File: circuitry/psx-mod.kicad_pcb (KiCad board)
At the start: 2 copper layers, 57 parts, among them J1 2x3P, J2 1x6P, J3 1x6P, J4 1x6P, J5 USB 2.0 Type-C, Q1 SI2302, Q2 SI2302, SW1 RESET, U1 TPS78318DDCT, U2 CDCE925PWR, U3 74HC04, U4 ATmega328P-A, U5 USBLC6-2SC6, U6 CH340G, Y1 16MHz, Y2 27MHz, Y3 12MHz

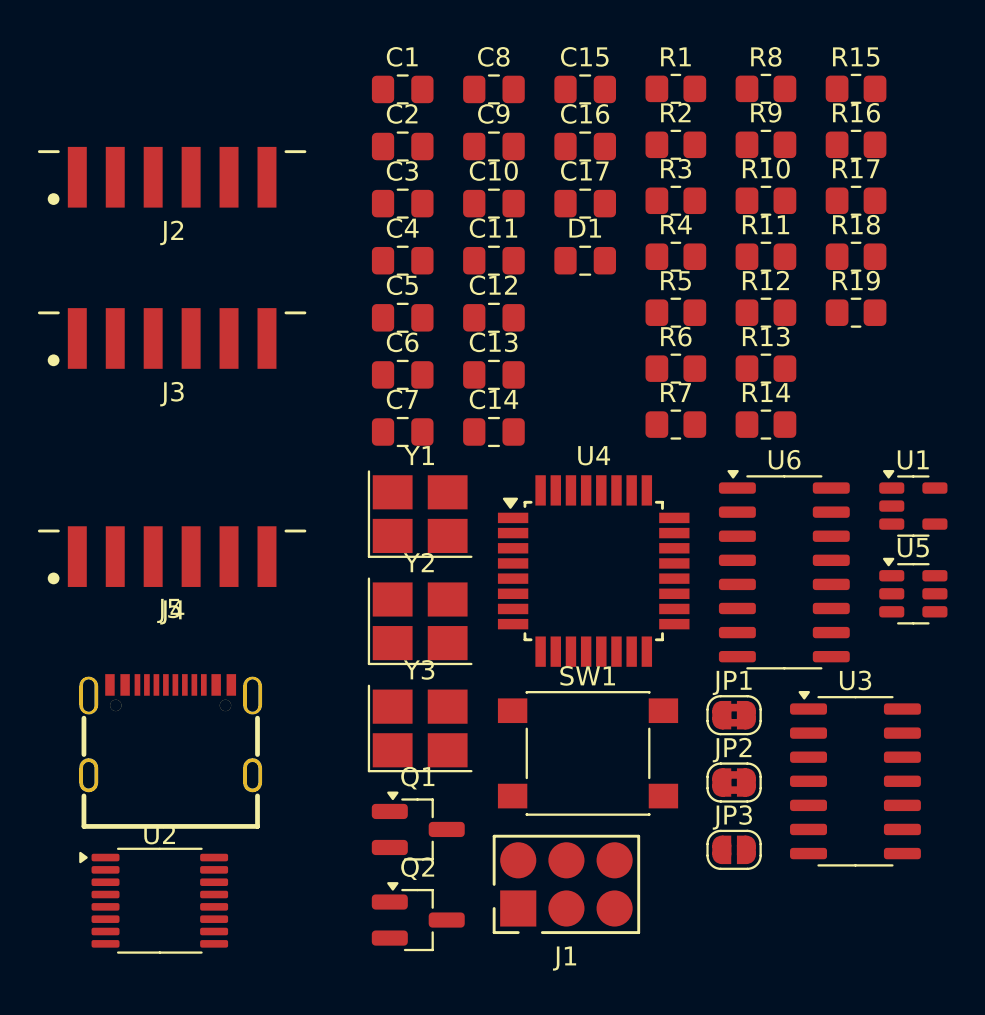
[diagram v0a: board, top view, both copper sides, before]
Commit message: Completed schematic and layout (badly).
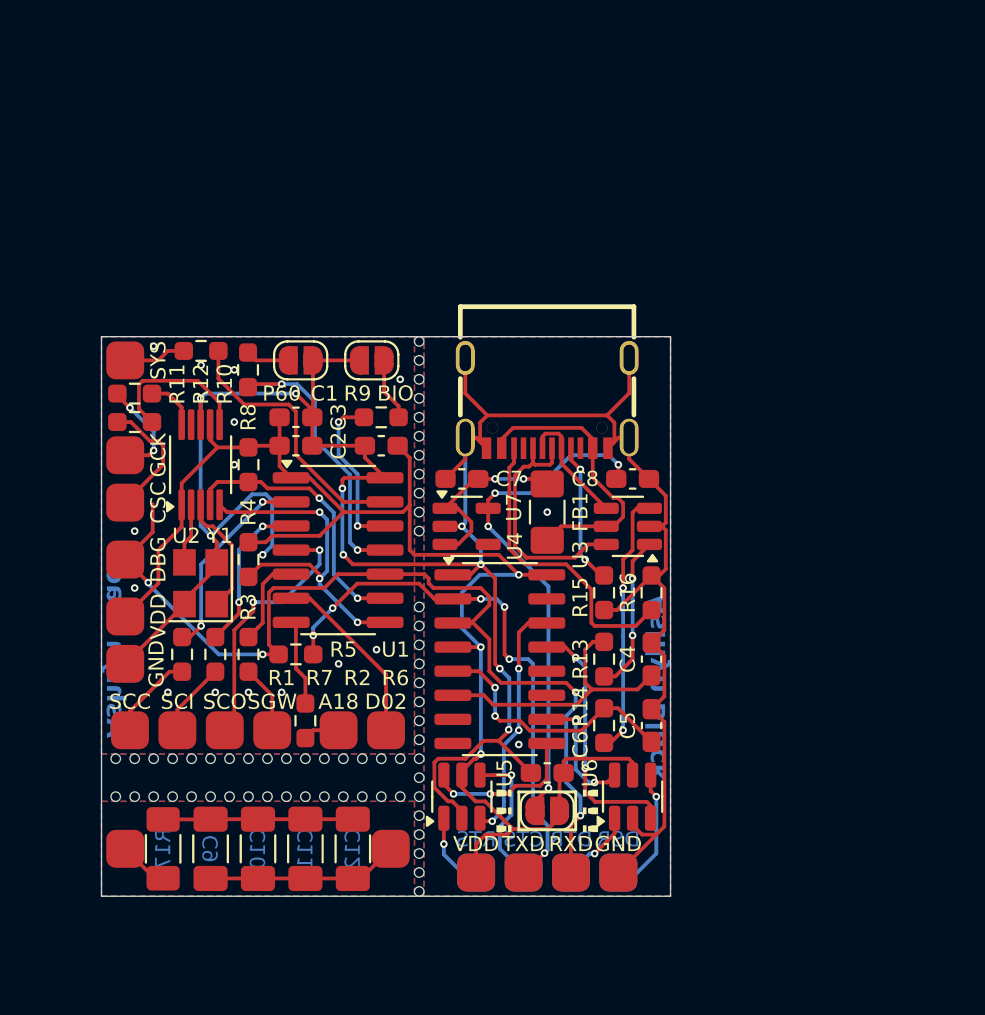
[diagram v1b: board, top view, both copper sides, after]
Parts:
- removed C13, C16: C, Capacitor_SMD:C_0805_2012Metric_Pad1.18x1.45mm_HandSolder
- removed C14, C15: 10pF, Capacitor_SMD:C_0805_2012Metric_Pad1.18x1.45mm_HandSolder
- removed C17: 100nF, Capacitor_SMD:C_0805_2012Metric_Pad1.18x1.45mm_HandSolder
- removed D1: RED, Capacitor_SMD:C_0805_2012Metric_Pad1.18x1.45mm_HandSolder
- removed J2, J3: 1x6P, PSX_Mod:CONN-PH 1x06_P2.00mm_Horizontal
- removed Q1, Q2: SI2302, Package_TO_SOT_SMD:SOT-23_Handsoldering
- removed R18, R19: 5.1kΩ, Resistor_SMD:R_0805_2012Metric_Pad1.20x1.40mm_HandSolder
- removed SW1: RESET, Button_Switch_SMD:SW_Push_1P1T_NO_6x6mm_H9.5mm
- removed Y2: 27MHz, Crystal:Crystal_SMD_3225-4Pin_3.2x2.5mm_HandSoldering
- removed Y3: 12MHz, Crystal:Crystal_SMD_3225-4Pin_3.2x2.5mm_HandSoldering
- added FB1: FerriteBead, Inductor_SMD:L_1206_3216Metric_Pad1.42x1.75mm_HandSolder, F.Cu at (158.8, 98.0)
- added J10: USB 2.0 Type-C, PSX_Mod:CONN-SMD_HX-TYPE-C-16PIN, F.Cu at (158.8, 92.2)
- added J11: Conn_01x04, PSX_Mod:CONN-SMD_4P, B.Cu at (158.8, 117.0)
- added J12: Conn_01x01, PSX_Mod:CONN-SMD_1P, F.Cu at (136.5, 115.8)
- added J13: Conn_01x01, PSX_Mod:CONN-SMD_1P, F.Cu at (150.5, 115.8)
- added J6: Conn_01x01, PSX_Mod:CONN-SMD_1P, F.Cu at (136.5, 100.5)
- added J7: Conn_01x01, PSX_Mod:CONN-SMD_1P, F.Cu at (136.5, 90.0)
- added J8: Conn_01x02, PSX_Mod:CONN-SMD_2P, F.Cu at (136.5, 96.2)
- added J9: Conn_01x04, PSX_Mod:CONN-SMD_4P, F.Cu at (158.8, 117.0)
- added REF**: MouseBite, PSX_Mod:MouseBite, F.Cu at (141.0, 113.0)
- added REF**: MouseBite, PSX_Mod:MouseBite, F.Cu at (147.0, 113.0)
- added REF**: MouseBite, PSX_Mod:MouseBite, F.Cu at (152.0, 90.0)
- added REF**: MouseBite, PSX_Mod:MouseBite, F.Cu at (152.0, 115.0)
- added REF**: MouseBite, PSX_Mod:MouseBite, F.Cu at (152.0, 114.0)
- added REF**: MouseBite, PSX_Mod:MouseBite, F.Cu at (152.0, 112.0)
- added REF**: MouseBite, PSX_Mod:MouseBite, F.Cu at (149.0, 111.0)
- added REF**: MouseBite, PSX_Mod:MouseBite, F.Cu at (138.0, 111.0)
- added REF**: MouseBite, PSX_Mod:MouseBite, F.Cu at (137.0, 113.0)
- added REF**: MouseBite, PSX_Mod:MouseBite, F.Cu at (152.0, 92.0)
- added REF**: MouseBite, PSX_Mod:MouseBite, F.Cu at (152.0, 107.0)
- added REF**: MouseBite, PSX_Mod:MouseBite, F.Cu at (152.0, 105.0)
- added REF**: MouseBite, PSX_Mod:MouseBite, F.Cu at (152.0, 99.0)
- added REF**: MouseBite, PSX_Mod:MouseBite, F.Cu at (136.0, 113.0)
- added REF**: MouseBite, PSX_Mod:MouseBite, F.Cu at (148.0, 111.0)
- added REF**: MouseBite, PSX_Mod:MouseBite, F.Cu at (147.0, 111.0)
- added REF**: MouseBite, PSX_Mod:MouseBite, F.Cu at (137.0, 111.0)
- added REF**: MouseBite, PSX_Mod:MouseBite, F.Cu at (152.0, 98.0)
- added REF**: MouseBite, PSX_Mod:MouseBite, F.Cu at (152.0, 108.0)
- added REF**: MouseBite, PSX_Mod:MouseBite, F.Cu at (140.0, 111.0)
- added REF**: MouseBite, PSX_Mod:MouseBite, F.Cu at (152.0, 109.0)
- added REF**: MouseBite, PSX_Mod:MouseBite, F.Cu at (150.0, 111.0)
- added REF**: MouseBite, PSX_Mod:MouseBite, F.Cu at (152.0, 116.0)
- added REF**: MouseBite, PSX_Mod:MouseBite, F.Cu at (152.0, 106.0)
- added REF**: MouseBite, PSX_Mod:MouseBite, F.Cu at (142.0, 113.0)
- added REF**: MouseBite, PSX_Mod:MouseBite, F.Cu at (152.0, 93.0)
- added REF**: MouseBite, PSX_Mod:MouseBite, F.Cu at (148.0, 113.0)
- added REF**: MouseBite, PSX_Mod:MouseBite, F.Cu at (144.0, 113.0)
- added REF**: MouseBite, PSX_Mod:MouseBite, F.Cu at (141.0, 111.0)
- added REF**: MouseBite, PSX_Mod:MouseBite, F.Cu at (150.0, 113.0)
- added REF**: MouseBite, PSX_Mod:MouseBite, F.Cu at (146.0, 113.0)
- added REF**: MouseBite, PSX_Mod:MouseBite, F.Cu at (143.0, 111.0)
- added REF**: MouseBite, PSX_Mod:MouseBite, F.Cu at (146.0, 111.0)
- added REF**: MouseBite, PSX_Mod:MouseBite, F.Cu at (152.0, 111.0)
- added REF**: MouseBite, PSX_Mod:MouseBite, F.Cu at (144.0, 111.0)
- added REF**: MouseBite, PSX_Mod:MouseBite, F.Cu at (152.0, 95.0)
- added REF**: MouseBite, PSX_Mod:MouseBite, F.Cu at (152.0, 117.0)
- added REF**: MouseBite, PSX_Mod:MouseBite, F.Cu at (151.0, 113.0)
- added REF**: MouseBite, PSX_Mod:MouseBite, F.Cu at (139.0, 111.0)
- added REF**: MouseBite, PSX_Mod:MouseBite, F.Cu at (140.0, 113.0)
- added REF**: MouseBite, PSX_Mod:MouseBite, F.Cu at (149.0, 113.0)
- added REF**: MouseBite, PSX_Mod:MouseBite, F.Cu at (152.0, 118.0)
- added REF**: MouseBite, PSX_Mod:MouseBite, F.Cu at (152.0, 113.0)
- added REF**: MouseBite, PSX_Mod:MouseBite, F.Cu at (143.0, 113.0)
- added REF**: MouseBite, PSX_Mod:MouseBite, F.Cu at (152.0, 110.0)
- added REF**: MouseBite, PSX_Mod:MouseBite, F.Cu at (138.0, 113.0)
- added REF**: MouseBite, PSX_Mod:MouseBite, F.Cu at (152.0, 97.0)
- added REF**: MouseBite, PSX_Mod:MouseBite, F.Cu at (139.0, 113.0)
- added REF**: MouseBite, PSX_Mod:MouseBite, F.Cu at (152.0, 96.0)
- added REF**: MouseBite, PSX_Mod:MouseBite, F.Cu at (136.0, 111.0)
- added REF**: MouseBite, PSX_Mod:MouseBite, F.Cu at (145.0, 111.0)
- added REF**: MouseBite, PSX_Mod:MouseBite, F.Cu at (145.0, 113.0)
- added REF**: MouseBite, PSX_Mod:MouseBite, F.Cu at (152.0, 91.0)
- added REF**: MouseBite, PSX_Mod:MouseBite, F.Cu at (142.0, 111.0)
- added REF**: MouseBite, PSX_Mod:MouseBite, F.Cu at (152.0, 104.0)
- added REF**: MouseBite, PSX_Mod:MouseBite, F.Cu at (152.0, 94.0)
- added REF**: MouseBite, PSX_Mod:MouseBite, F.Cu at (151.0, 111.0)
- added REF**: MouseBite, PSX_Mod:MouseBite, F.Cu at (152.0, 103.0)
- added REF**: MouseBite, PSX_Mod:MouseBite, F.Cu at (152.0, 89.0)
- added U7: XC6219B332MR, Package_TO_SOT_SMD:SOT-23-5, F.Cu at (154.5, 98.8)
- C1, C3, C8: value 100nF -> 10µF; footprint Capacitor_SMD:C_0805_2012Metric_Pad1.18x1.45mm_HandSolder -> Capacitor_SMD:C_0603_1608Metric_Pad1.08x0.95mm_HandSolder
- C10: value C -> 47µF; footprint Capacitor_SMD:C_0805_2012Metric_Pad1.18x1.45mm_HandSolder -> Capacitor_SMD:C_1206_3216Metric_Pad1.33x1.80mm_HandSolder
- C11, C12, C9: value 100nF -> 47µF; footprint Capacitor_SMD:C_0805_2012Metric_Pad1.18x1.45mm_HandSolder -> Capacitor_SMD:C_1206_3216Metric_Pad1.33x1.80mm_HandSolder
- C2, C7: value 1µF -> 10µF; footprint Capacitor_SMD:C_0805_2012Metric_Pad1.18x1.45mm_HandSolder -> Capacitor_SMD:C_0603_1608Metric_Pad1.08x0.95mm_HandSolder
- C4: value 100nF -> 10pF; footprint Capacitor_SMD:C_0805_2012Metric_Pad1.18x1.45mm_HandSolder -> Capacitor_SMD:C_0603_1608Metric_Pad1.08x0.95mm_HandSolder
- C5: value 1µF -> 10pF; footprint Capacitor_SMD:C_0805_2012Metric_Pad1.18x1.45mm_HandSolder -> Capacitor_SMD:C_0603_1608Metric_Pad1.08x0.95mm_HandSolder
- C6: value C -> 10µF; footprint Capacitor_SMD:C_0805_2012Metric_Pad1.18x1.45mm_HandSolder -> Capacitor_SMD:C_0603_1608Metric_Pad1.08x0.95mm_HandSolder
- J1: value 2x3P -> Conn_01x04; footprint PSX_Mod:CONN-SMD_POGO-ISP -> PSX_Mod:CONN-SMD_4P
- J4: value 1x6P -> Conn_01x02; footprint PSX_Mod:CONN-PH 1x06_P2.00mm_Horizontal -> PSX_Mod:CONN-SMD_2P
- J5: value USB 2.0 Type-C -> Conn_01x02; footprint PSX_Mod:CONN-SMD_HX-TYPE-C-16PIN -> PSX_Mod:CONN-SMD_2P
- JP1, JP2: value SolderJumper_2_Bridged -> JMP2O; footprint Jumper:SolderJumper-2_P1.3mm_Bridged2Bar_RoundedPad1.0x1.5mm -> Jumper:SolderJumper-2_P1.3mm_Open_RoundedPad1.0x1.5mm
- JP3: value SolderJumper_2_Open -> Jumper_2_Open
- R1: value 1kΩ -> 10kΩ; footprint Resistor_SMD:R_0805_2012Metric_Pad1.20x1.40mm_HandSolder -> Resistor_SMD:R_0603_1608Metric_Pad0.98x0.95mm_HandSolder
- R10: value 18Ω -> 10kΩ; footprint Resistor_SMD:R_0805_2012Metric_Pad1.20x1.40mm_HandSolder -> Resistor_SMD:R_0603_1608Metric_Pad0.98x0.95mm_HandSolder
- R11: value 10kΩ -> 220Ω; footprint Resistor_SMD:R_0805_2012Metric_Pad1.20x1.40mm_HandSolder -> Resistor_SMD:R_0603_1608Metric_Pad0.98x0.95mm_HandSolder
- R12: value 1kΩ -> 2.2kΩ; footprint Resistor_SMD:R_0805_2012Metric_Pad1.20x1.40mm_HandSolder -> Resistor_SMD:R_0603_1608Metric_Pad0.98x0.95mm_HandSolder
- R13, R14: value 1kΩ -> 10Ω; footprint Resistor_SMD:R_0805_2012Metric_Pad1.20x1.40mm_HandSolder -> Resistor_SMD:R_0603_1608Metric_Pad0.98x0.95mm_HandSolder
- R15: value 18Ω -> 5.1kΩ; footprint Resistor_SMD:R_0805_2012Metric_Pad1.20x1.40mm_HandSolder -> Resistor_SMD:R_0603_1608Metric_Pad0.98x0.95mm_HandSolder
- R16: value 10Ω -> 5.1kΩ; footprint Resistor_SMD:R_0805_2012Metric_Pad1.20x1.40mm_HandSolder -> Resistor_SMD:R_0603_1608Metric_Pad0.98x0.95mm_HandSolder
- R17: value 10Ω -> 75Ω; footprint Resistor_SMD:R_0805_2012Metric_Pad1.20x1.40mm_HandSolder -> Resistor_SMD:R_1206_3216Metric_Pad1.30x1.75mm_HandSolder
- R2, R3, R4, R6, R9: footprint Resistor_SMD:R_0805_2012Metric_Pad1.20x1.40mm_HandSolder -> Resistor_SMD:R_0603_1608Metric_Pad0.98x0.95mm_HandSolder
- R5: value 10kΩ -> 4.7kΩ; footprint Resistor_SMD:R_0805_2012Metric_Pad1.20x1.40mm_HandSolder -> Resistor_SMD:R_0603_1608Metric_Pad0.98x0.95mm_HandSolder
- R7, R8: value 100Ω -> 10kΩ; footprint Resistor_SMD:R_0805_2012Metric_Pad1.20x1.40mm_HandSolder -> Resistor_SMD:R_0603_1608Metric_Pad0.98x0.95mm_HandSolder
- U1: value TPS78318DDCT -> ATtiny404-SS; footprint Package_TO_SOT_SMD:SOT-23-5 -> Package_SO:SOIC-14_3.9x8.7mm_P1.27mm
- U2: value CDCE925PWR -> Si5351A-B-GT; footprint Package_SO:TSSOP-16_4.4x5mm_P0.65mm -> Package_SO:MSOP-10_3x3mm_P0.5mm
- U3: value 74HC04 -> USBLC6-2SC6; footprint Package_SO:SOIC-14_3.9x8.7mm_P1.27mm -> Package_TO_SOT_SMD:SOT-23-6
- U4: value ATmega328P-A -> CH340C; footprint Package_QFP:TQFP-32_7x7mm_P0.8mm -> Package_SO:SOIC-16_3.9x9.9mm_P1.27mm
- U5: value USBLC6-2SC6 -> 74LVC2G04
- U6: value CH340G -> 74LVC2G04; footprint Package_SO:SOIC-16_3.9x9.9mm_P1.27mm -> Package_TO_SOT_SMD:SOT-23-6
- Y1: value 16MHz -> 27MHz; footprint Crystal:Crystal_SMD_3225-4Pin_3.2x2.5mm_HandSoldering -> Crystal:Crystal_SMD_3225-4Pin_3.2x2.5mm
- moved R17 50.0 mm to (138.5, 115.8), turned to -90 degrees
- moved C9 39.9 mm to (141.0, 115.8), turned to 90 degrees
- moved R1 39.6 mm to (139.5, 105.5), turned to -90 degrees
- moved C10 36.2 mm to (143.5, 115.8), turned to 90 degrees
- moved R2 36.2 mm to (141.3, 105.5), turned to -90 degrees
- moved R11 34.1 mm to (137.0, 91.8), turned to 180 degrees
- moved R12 33.8 mm to (137.0, 93.2), turned to 180 degrees
- moved C11 32.6 mm to (146.0, 115.8), turned to 90 degrees
- moved R8 31.1 mm to (143.0, 90.5), turned to 90 degrees
- moved R10 30.8 mm to (140.5, 89.5), turned to 180 degrees
- moved U1 30.4 mm to (147.8, 100.0)
- moved R15 29.7 mm to (161.8, 102.2), turned to -90 degrees
- moved JP1 29.5 mm to (145.8, 90.0)
- moved R3 29.4 mm to (143.0, 100.5), turned to -90 degrees
- moved JP2 29.3 mm to (149.5, 90.0), turned to 180 degrees
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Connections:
- C1 pad 1: +3V3 -> VDD
- C10 pad 1: GND -> Net-(J13-Pin_1)
- C10 pad 2: Net-(U4-XTAL2/PB7) -> Net-(C10-Pad2)
- C11 pad 1: +3V3 -> Net-(J13-Pin_1)
- C11 pad 2: GND -> Net-(C10-Pad2)
- C12 pad 1: +3V3 -> Net-(J13-Pin_1)
- C12 pad 2: GND -> Net-(C10-Pad2)
- C2 pad 1: +3V3 -> VDD
- C3 pad 1: +3V3 -> VDD
- C4 pad 1: +1V8 -> Net-(U4-UD-)
- C5 pad 1: +1V8 -> Net-(U4-UD+)
- C6 pad 1: GND -> VDD
- C6 pad 2: Net-(U4-XTAL1/PB6) -> GND
- C7 pad 1: +3V3 -> Net-(U7-CE)
- C8 pad 1: +3V3 -> Net-(JP3-A)
- C9 pad 1: +3V3 -> Net-(J13-Pin_1)
- C9 pad 2: GND -> Net-(C10-Pad2)
- J1 pad 1: /MISO -> /scc
- J1 pad 2: +3V3 -> /sci
- J1 pad 3: /SCLK -> /sco
- J1 pad 4: /MOSI -> /sgw
- J4 pad 1: /RXD -> /d02
- J4 pad 2: /TXD -> /a18
- JP1 pad 1: /RXD -> /~{p60}
- JP1 pad 2: ARX -> GND
- JP2 pad 1: /TXD -> /~{rom}
- JP2 pad 2: ATX -> GND
- JP3 pad 2: Net-(JP3-B) -> VDD
- R1 pad 1: Net-(D1-K) -> Net-(U1-PA4)
- R1 pad 2: Net-(U4-PB2) -> /scc
- R10 pad 1: Net-(U2-Y2) -> Net-(U1-PA3)
- R10 pad 2: /PSX_CLK1 -> /sys
- R11 pad 1: Net-(U2-S0) -> Net-(U2-CLK0)
- R11 pad 2: GND -> /gck
- R12 pad 1: Net-(U4-PB0) -> Net-(U2-CLK2)
- R12 pad 2: /DATA -> /csc
- R13 pad 1: ARX -> Net-(R13-Pad1)
- R13 pad 2: Net-(U4-PD0) -> Net-(U4-UD-)
- R14 pad 1: Net-(U4-PB1) -> Net-(R14-Pad1)
- R14 pad 2: /GATE -> Net-(U4-UD+)
- R15 pad 1: Net-(U2-Y5) -> Net-(J10-CC1)
- R15 pad 2: /PSX_CLK2 -> GND
- R16 pad 1: Net-(R16-Pad1) -> Net-(J10-CC2)
- R16 pad 2: Net-(U6-UD+) -> GND
- R17 pad 1: Net-(R17-Pad1) -> Net-(C10-Pad2)
- R17 pad 2: Net-(U6-UD-) -> Net-(J12-Pin_1)
- R2 pad 1: +3V3 -> Net-(U1-PA5)
- R2 pad 2: ~{RST} -> /sci
- R3 pad 1: +1V8 -> VDD
- R3 pad 2: Net-(Q1-S) -> Net-(U1-PB1)
- R4 pad 1: +1V8 -> VDD
- R4 pad 2: Net-(Q2-S) -> Net-(U1-PB0)
- R5 pad 1: +3V3 -> /txd
- R5 pad 2: SDA -> /dbg
- R6 pad 1: +3V3 -> Net-(U1-PA7)
- R6 pad 2: SCL -> /sgw
- R7 pad 1: Net-(U2-SDA/S1) -> Net-(U1-PB2)
- R7 pad 2: Net-(Q1-S) -> /a18
- R8 pad 1: Net-(U2-SCL/S2) -> Net-(U1-PA1)
- R8 pad 2: Net-(Q2-S) -> /~{p60}
- R9 pad 1: Net-(U2-S0) -> Net-(U1-PA2)
- R9 pad 2: /~{PSX_PAL} -> /~{rom}
- U1 pad 1: +3V3 -> VDD
- U1 pad 2: GND -> Net-(U1-PA4)
- U1 pad 3: +3V3 -> Net-(U1-PA5)
- U1 pad 4: GND -> /sco
- U1 pad 5: +1V8 -> Net-(U1-PA7)
- U2 pad 1: Net-(U2-XIN/CLK) -> VDD
- U2 pad 10: unconnected-(U2-Y3-Pad10) -> Net-(U2-CLK0)
- U2 pad 2: Net-(U2-S0) -> Net-(U2-XA)
- U2 pad 3: +1V8 -> Net-(U2-XB)
- U2 pad 4: unconnected-(U2-VCTRL-Pad4) -> Net-(U1-PB0)
- U2 pad 5: GND -> Net-(U1-PB1)
- U2 pad 6: +3V3 -> Net-(U2-CLK2)
- U2 pad 7: unconnected-(U2-Y4-Pad7) -> VDD
- U2 pad 8: Net-(U2-Y5) -> GND
- U2 pad 9: +3V3 -> unconnected-(U2-CLK1-Pad9)
- U3 pad 1: /RTS -> Net-(R13-Pad1)
- U3 pad 2: Net-(U6-~{CTS}) -> GND
- U3 pad 3: Net-(U6-~{RTS}) -> Net-(R14-Pad1)
- U3 pad 4: /CTS -> Net-(J10-D--PadA7)
- U3 pad 5: /DTR -> VBUS
- U3 pad 6: Net-(U6-~{DSR}) -> Net-(J10-D+-PadA6)
- U4 pad 1: unconnected-(U4-PD3-Pad1) -> GND
- U4 pad 10: /SQCK -> Net-(U4-~{DSR})
- U4 pad 11: /SUBQ -> unconnected-(U4-~{RI}-Pad11)
- U4 pad 12: Net-(U4-PB0) -> unconnected-(U4-~{DCD}-Pad12)
- U4 pad 13: Net-(U4-PB1) -> Net-(U4-~{DTR})
- U4 pad 14: Net-(U4-PB2) -> Net-(U4-~{RTS})
- U4 pad 15: /MOSI -> unconnected-(U4-R232-Pad15)
- U4 pad 16: /MISO -> VDD
- U4 pad 2: /A18 -> /txd
- U4 pad 3: GND -> /dbg
- U4 pad 4: +3V3 -> VDD
- U4 pad 5: GND -> Net-(U4-UD+)
- U4 pad 6: +3V3 -> Net-(U4-UD-)
- U4 pad 7: Net-(U4-XTAL1/PB6) -> unconnected-(U4-NC-Pad7)
- U4 pad 8: Net-(U4-XTAL2/PB7) -> unconnected-(U4-~{OUT}-Pad8)
- U4 pad 9: /D2 -> Net-(U4-~{CTS})
- U5 pad 1: Net-(R16-Pad1) -> /rts
- U5 pad 3: Net-(R17-Pad1) -> Net-(U4-~{RTS})
- U5 pad 4: Net-(J5-D--PadA7) -> /cts
- U5 pad 5: Net-(U5-VBUS) -> VDD
- U5 pad 6: Net-(J5-D+-PadA6) -> Net-(U4-~{CTS})
- U6 pad 1: GND -> /dtr
- U6 pad 2: /RXD -> GND
- U6 pad 3: /TXD -> Net-(U4-~{DTR})
- U6 pad 4: +3V3 -> /dsr
- U6 pad 5: Net-(U6-UD+) -> VDD
- U6 pad 6: Net-(U6-UD-) -> Net-(U4-~{DSR})
- Y1 pad 1: Net-(U4-XTAL1/PB6) -> Net-(U2-XB)
- Y1 pad 3: Net-(U4-XTAL2/PB7) -> Net-(U2-XA)
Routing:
- net GND: track 0.00 -> 142.8 mm, vias 0 -> 26
- net VDD: track 0.00 -> 79.0 mm, vias 0 -> 3
- net /dbg: track 0.00 -> 51.8 mm, vias 0 -> 4
- net /txd: track 0.00 -> 29.3 mm, vias 0 -> 6
- net Net-(JP3-A): track 0.00 -> 27.0 mm, vias 0 -> 4
- net Net-(U1-PB1): track 0.00 -> 18.3 mm, vias 0 -> 3
- net Net-(J10-CC2): track 0.00 -> 16.0 mm
- net VBUS: track 0.00 -> 15.2 mm
- net Net-(U4-UD-): track 0.00 -> 14.7 mm
- net Net-(U1-PB0): track 0.00 -> 14.6 mm, vias 0 -> 2
- net Net-(U1-PA1): track 0.00 -> 14.3 mm, vias 0 -> 2
- net Net-(U1-PA3): track 0.00 -> 14.3 mm
- net /sco: track 0.00 -> 13.9 mm, vias 0 -> 2
- net Net-(R14-Pad1): track 0.00 -> 13.9 mm, vias 0 -> 2
- net Net-(U4-UD+): track 0.00 -> 13.9 mm, vias 0 -> 2
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- added copper zone on B.Cu, net (none)
- added copper zone on F.Cu, net (none)
- added copper zone on B.Cu, net GND
- added copper zone on F.Cu, net GND
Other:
- board outline added: 30 x 29.5 mm
- board text added: "!!!"
- board text added: "A18"
- board text added: "Ashlyn Black"
- board text added: "BIO"
- board text added: "CSC"
- board text added: "CTS"
- board text added: "D02"
- board text added: "DBG"
- board text added: "DSR"
- board text added: "DTR"
- board text added: "GCK"
- board text added: "GND"
- board text added: "P60"
- board text added: "RTS"
- board text added: "RXD"
- board text added: "SCC"
- board text added: "SCI"
- board text added: "SCO"
- board text added: "SGW"
- board text added: "SYS"
- board text added: "TXD"
- board text added: "VDD"
